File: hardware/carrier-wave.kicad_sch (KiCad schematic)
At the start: 4 parts, among them U2 OPA695, U3 THS3491, U4 AD9834, U7 TS5A3159ADCK

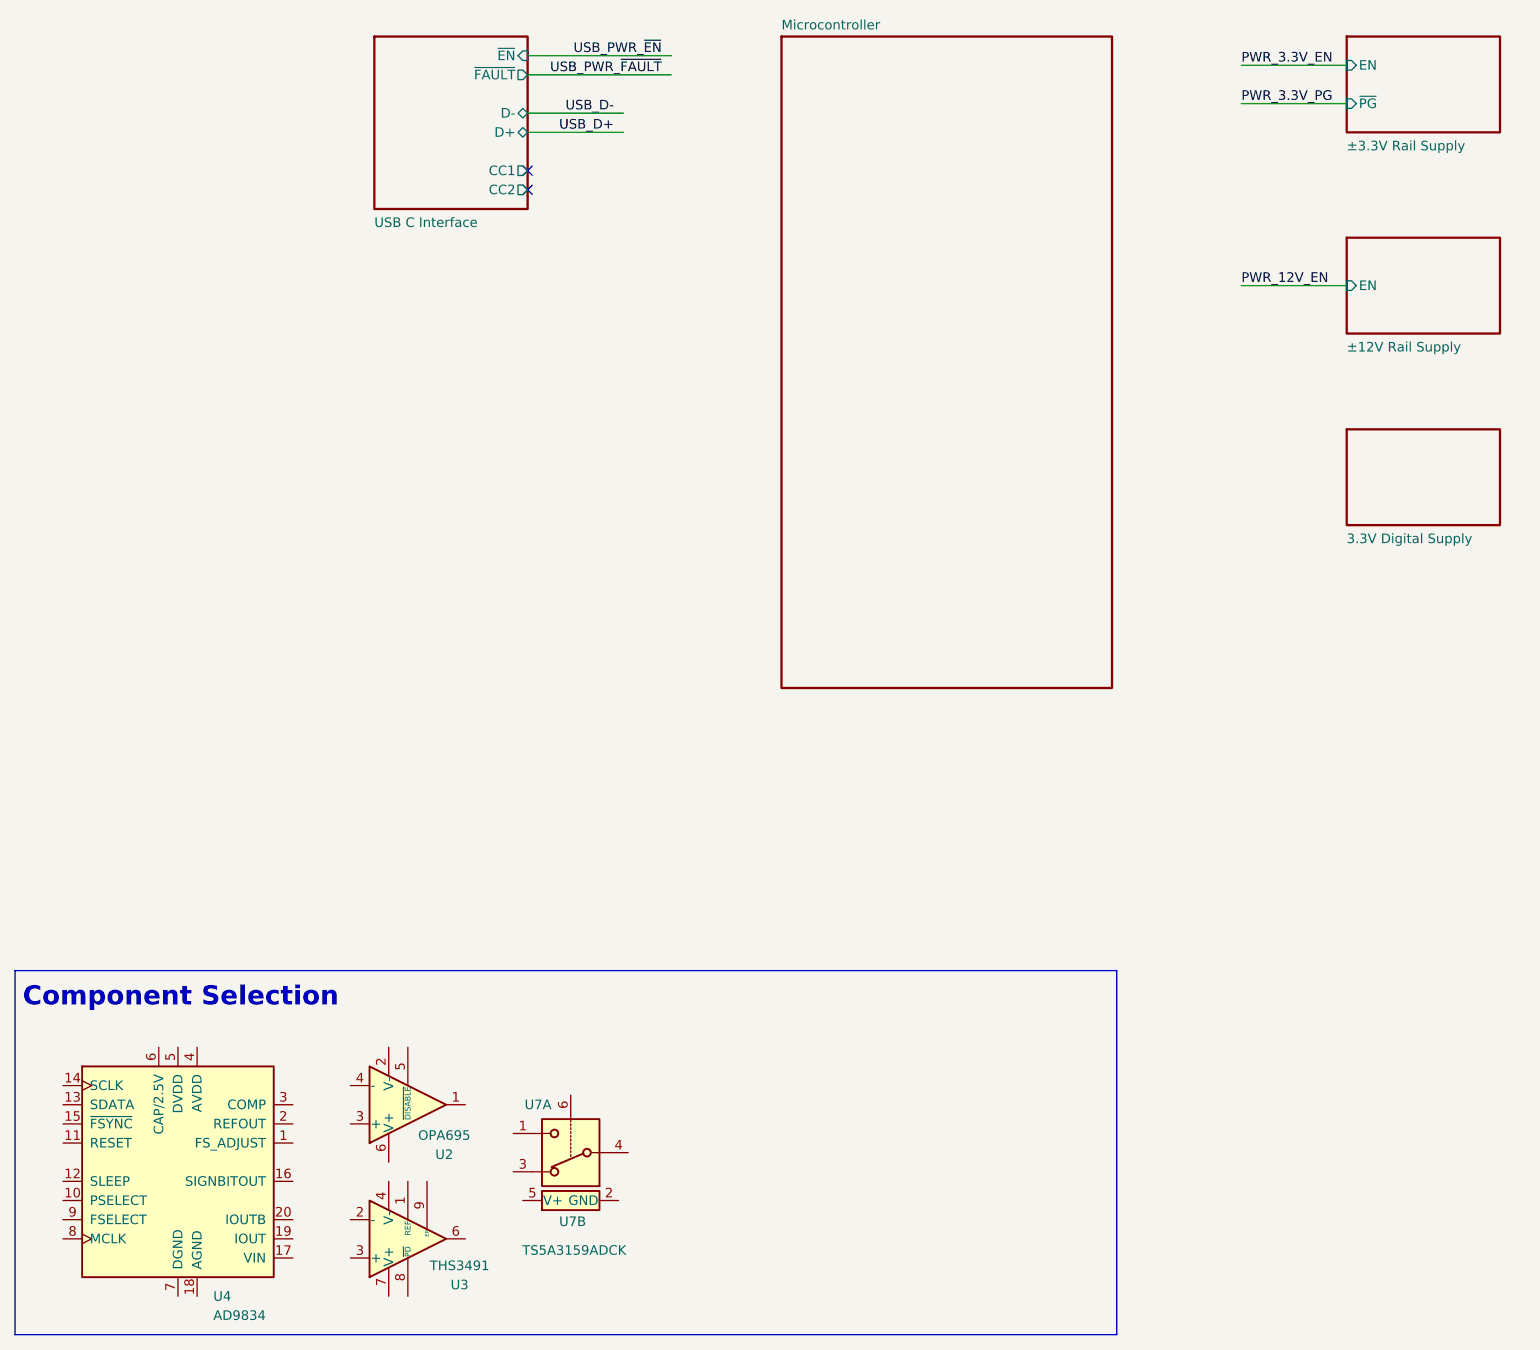
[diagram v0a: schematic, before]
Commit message: Cleanup Sheets
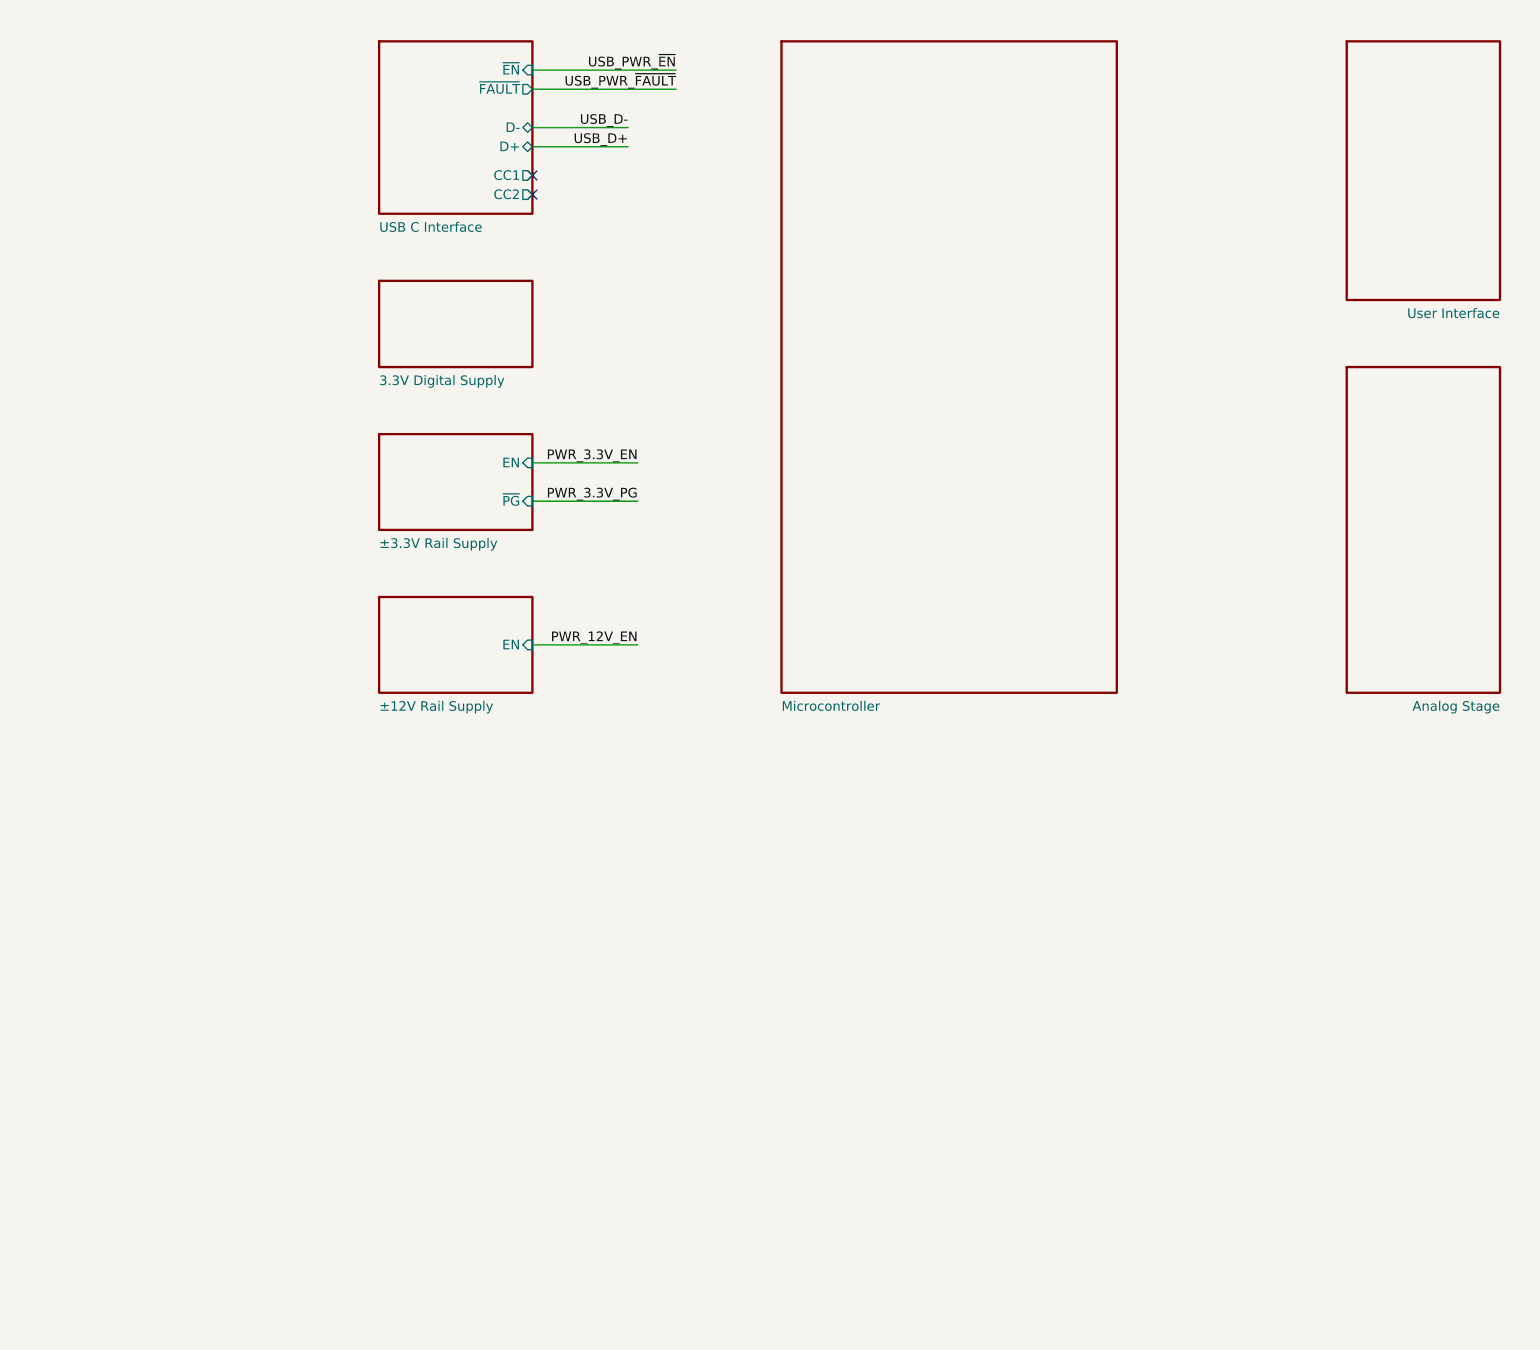
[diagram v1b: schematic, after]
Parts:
- removed U2: OPA695, Package_TO_SOT_SMD:SOT-23-6, symbol carrier-wave:OPA695
- removed U3: THS3491, Package_SO:Texas_R-PDSO-G8_EP2.95x4.9mm_Mask2.4x3.1mm_ThermalVias, symbol Amplifier_Operational:THS3491xDDA
- removed U4: AD9834, Package_SO:TSSOP-20_4.4x6.5mm_P0.65mm, symbol Interface:AD9834
- removed U7: TS5A3159ADCK, Package_TO_SOT_SMD:SOT-363_SC-70-6, symbol Analog_Switch:TS5A3159ADCK
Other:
- added sheet Analog Stage (analog-stage.kicad_sch)
- added sheet User Interface (user-interface.kicad_sch)
- note removed: "Component Selection"
